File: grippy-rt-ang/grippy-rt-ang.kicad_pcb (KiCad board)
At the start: 2 copper layers, 35.2 x 60.8 mm, 9 parts, among them J1 Conn_01x08_Socket, SW0 SW_SPST, SW1 SW_SPST, SW2 SW_SPST, SW3 SW_SPST, SW4 SW_SPST, SW5 SW_DPDT_x2, U1 esp32s3-supermini

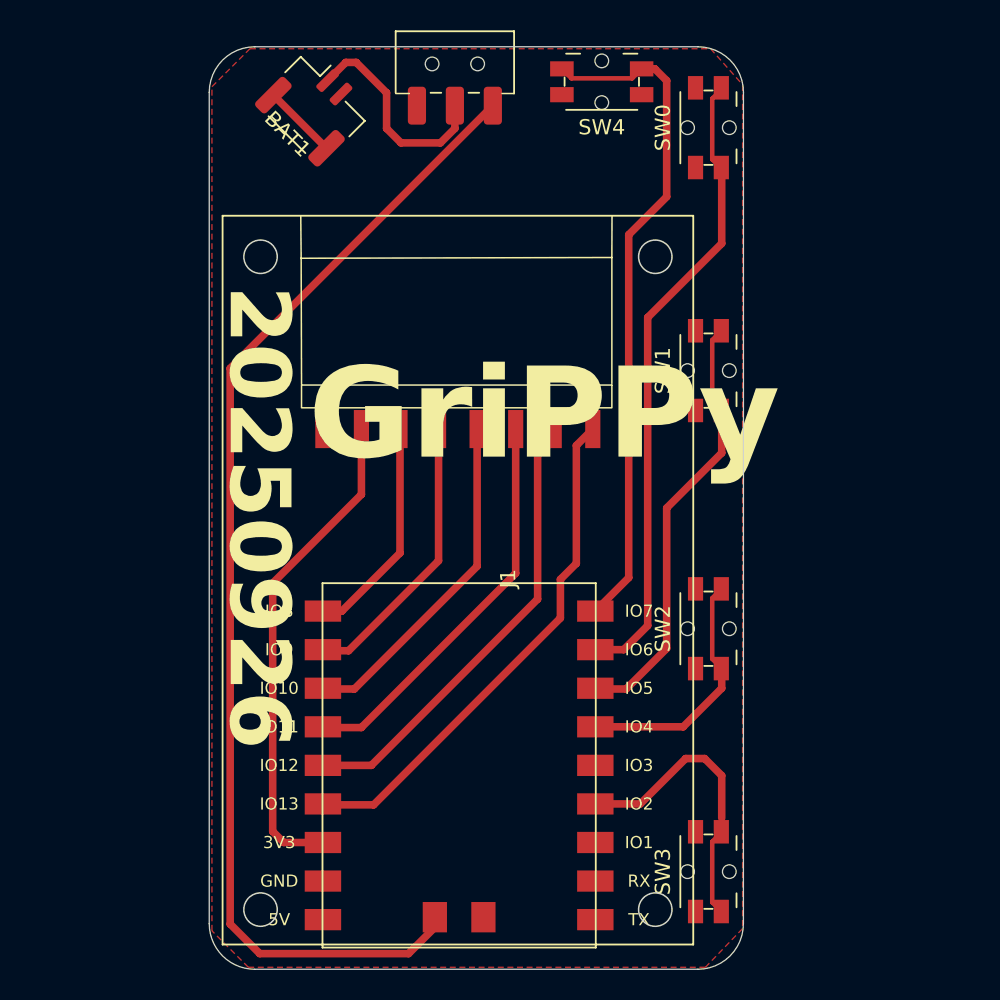
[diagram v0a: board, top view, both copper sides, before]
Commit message: new rt ang pcb stable started case
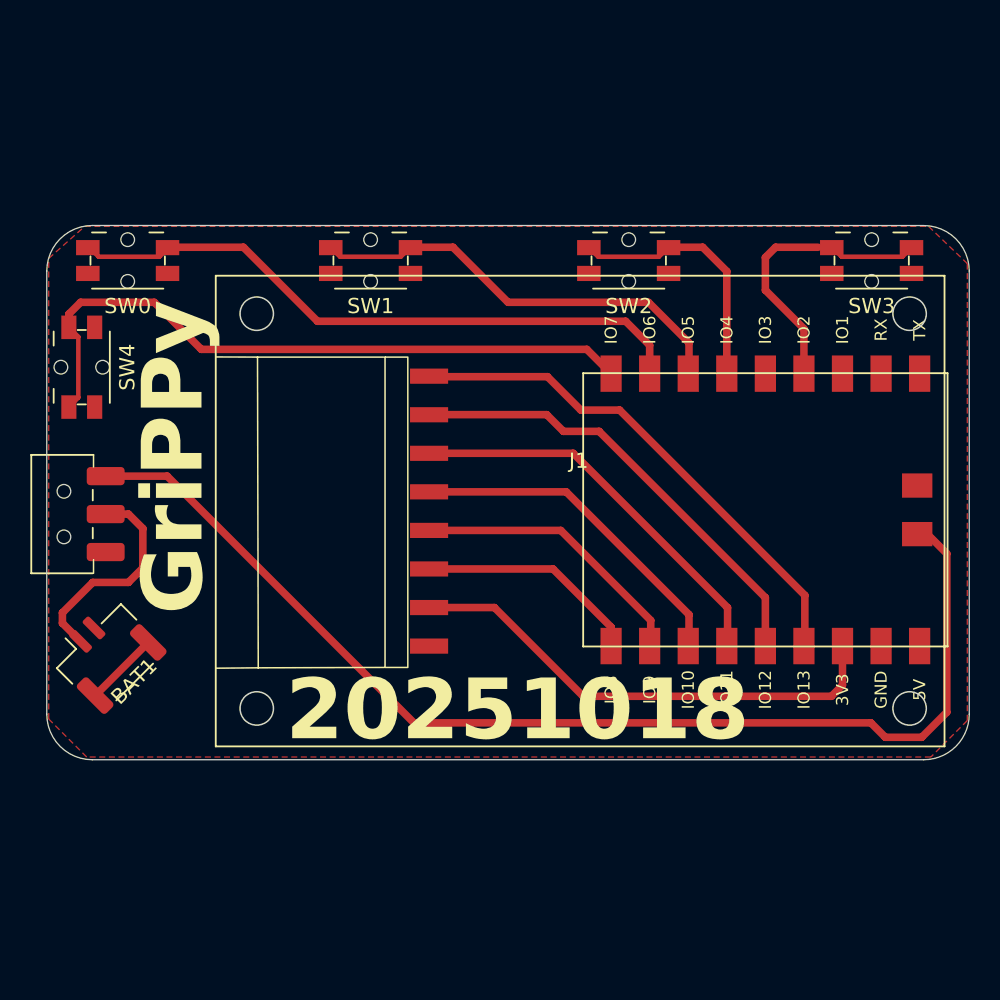
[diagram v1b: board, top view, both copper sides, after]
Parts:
- moved SW3 41.7 mm to (231.2, 69.0), turned to 0 degrees
- moved SW0 39.2 mm to (182.2, 69.0), turned to 0 degrees
- moved SW4 39.1 mm to (179.2, 76.0), turned to 90 degrees
- moved SW5 38.9 mm to (178.2, 85.7), turned to -90 degrees
- moved BAT1 38.5 mm to (180.9, 95.0), turned to 45 degrees
- moved U1 26.3 mm to (224.2, 85.4), turned to 90 degrees
- moved SW2 24.8 mm to (215.2, 69.0), turned to 0 degrees
- moved SW1 23.4 mm to (198.2, 69.0), turned to 0 degrees
- moved J1 9.25 mm to (212.0, 85.5), turned to 0 degrees
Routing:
- net /RAW: track 76.7 -> 76.1 mm
- net /ring: track 16.4 -> 16.9 mm
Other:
- board size 35.2 x 60.8 mm -> 60.8 x 35.2 mm
- board text added: "20251018"
- board text removed: "20250926"
